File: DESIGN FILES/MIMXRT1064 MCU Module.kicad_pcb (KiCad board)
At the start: 6 copper layers, 60 x 22 mm, 70 parts, among them J601 TF-15x15, U401 MIMXRT1064CVL5B, U601 IS25WP064A-JBLE, U602 IS42S16160J-6BLI, U701 M.2-B-KEY, Y401 7V24000026, Y402 Q13FC1350000200

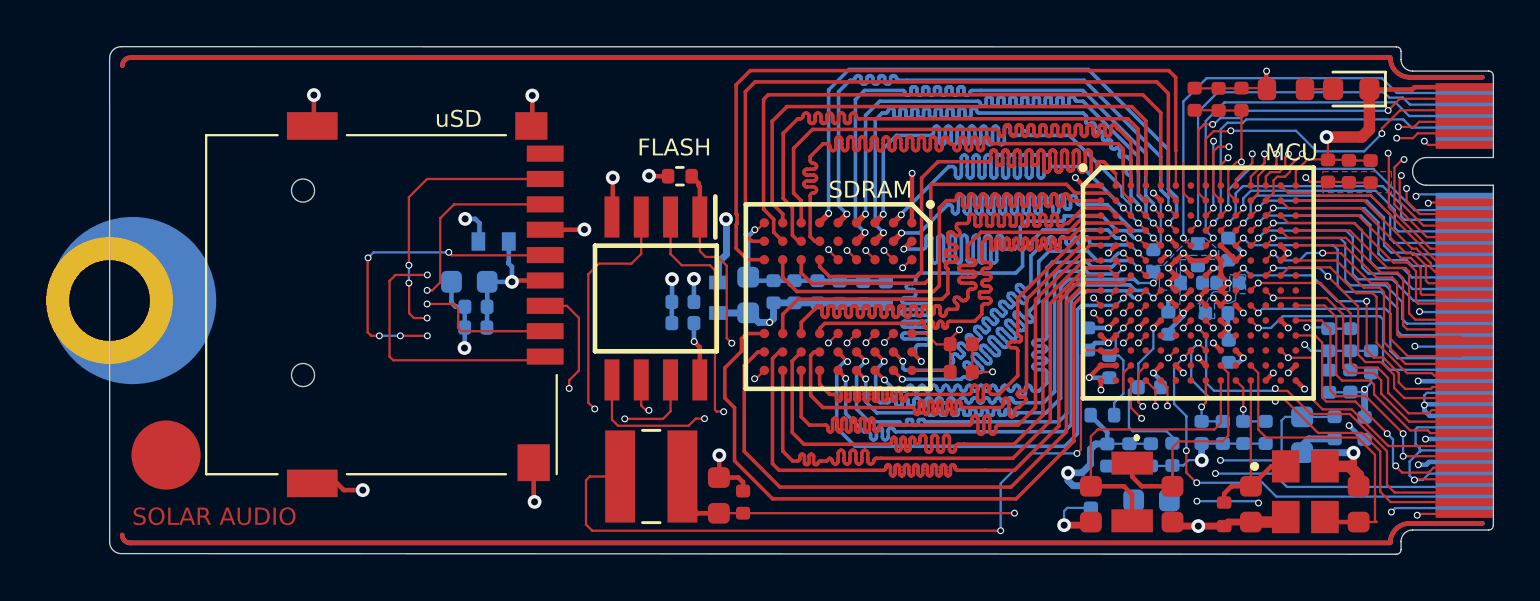
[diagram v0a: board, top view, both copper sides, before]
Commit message: up
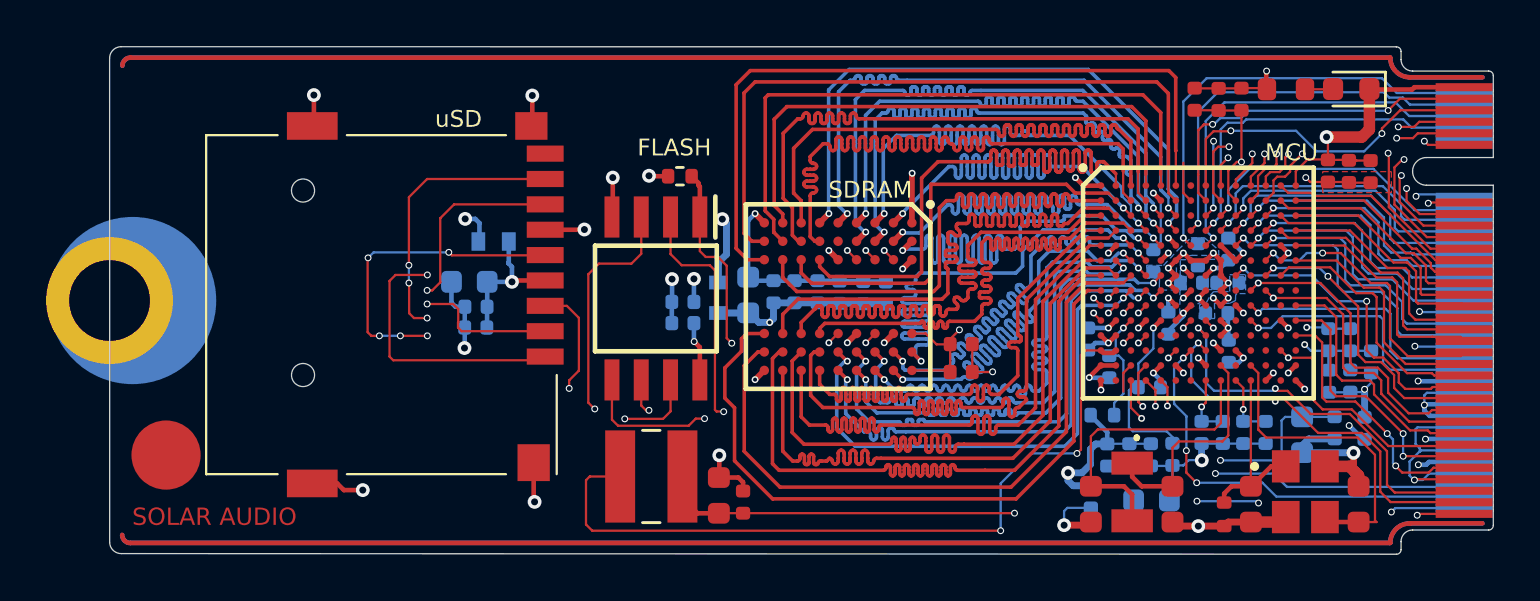
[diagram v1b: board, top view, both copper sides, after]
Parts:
- U602: value IS42S16160J-6BLI -> BGA54C80P9X9_800X800X120
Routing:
- net GND: track 124.9 -> 125.7 mm
